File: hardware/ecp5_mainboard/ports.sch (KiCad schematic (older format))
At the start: 97 parts, among them J13 Micro_SD_Card, J3 HDMI_A, J4 USB_A, P4 JK0654219NL, U17 TPS2041B, U18 PCA9306, U19 TFP410, U20 TPS2041B, U21 KSZ9031RNXCA, U22 USB3300-EZK, Y2 25MHz, Y3 24MHz

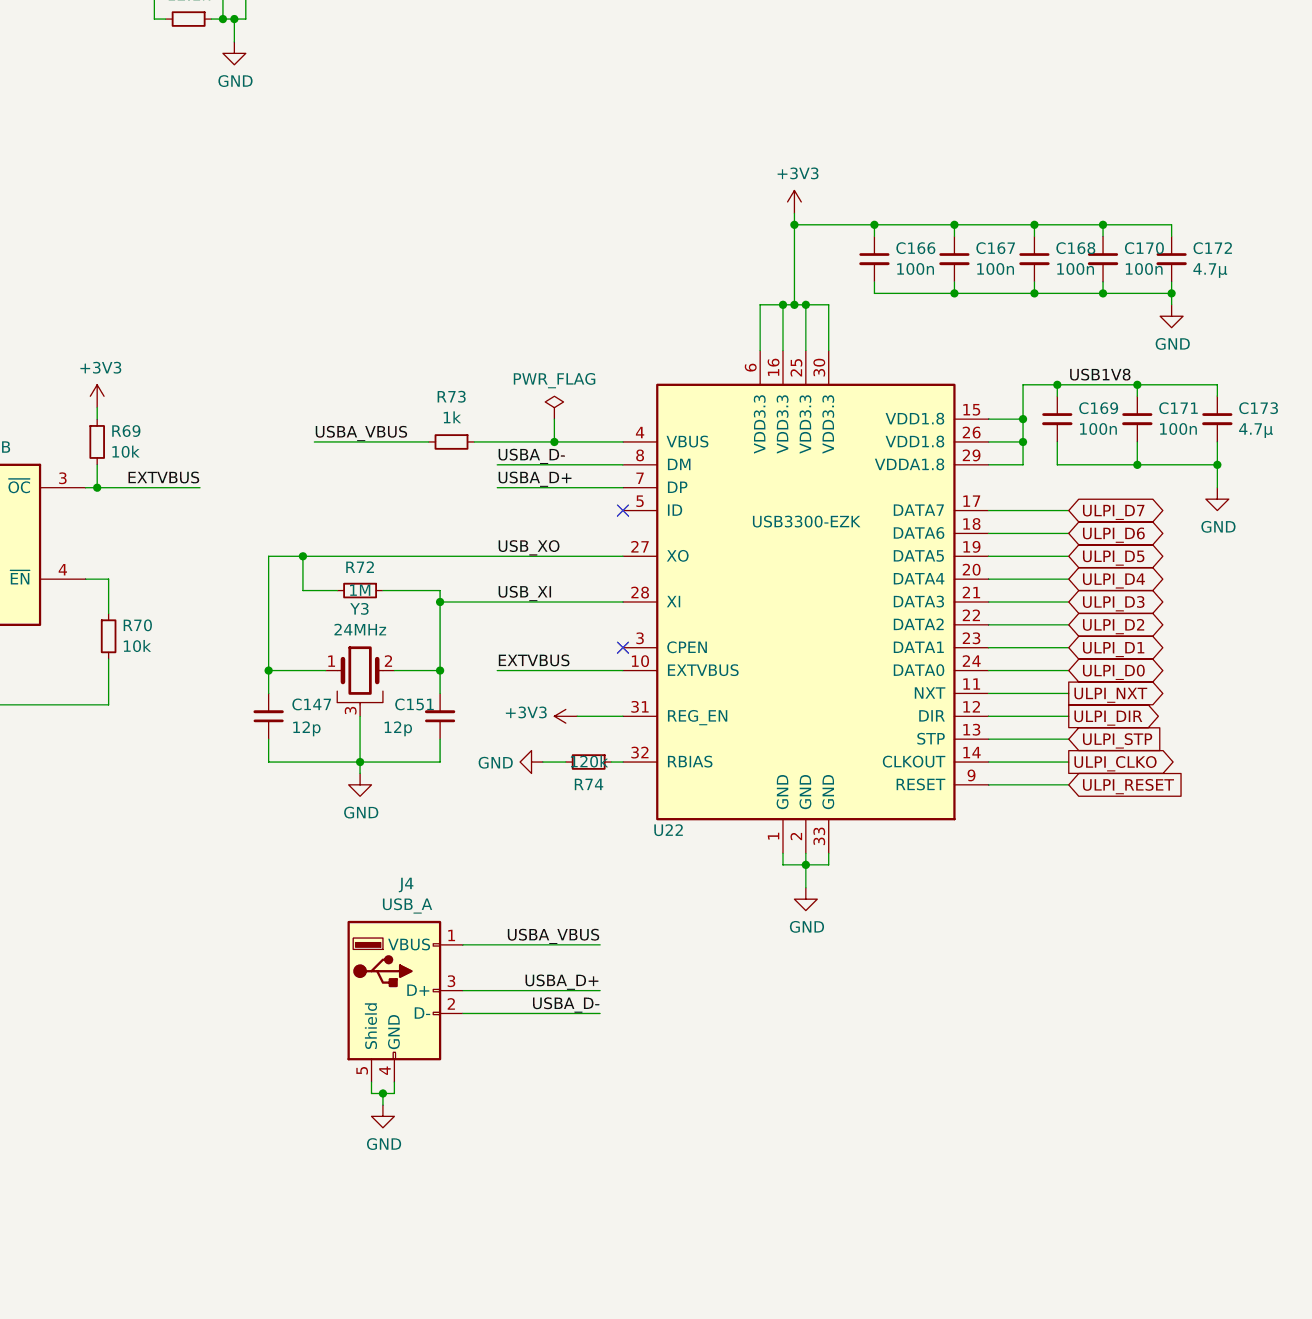
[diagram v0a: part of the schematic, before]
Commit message: hardware/mainboard: ERC fixes
Signed-off-by: David Shah <dave@ds0.me>
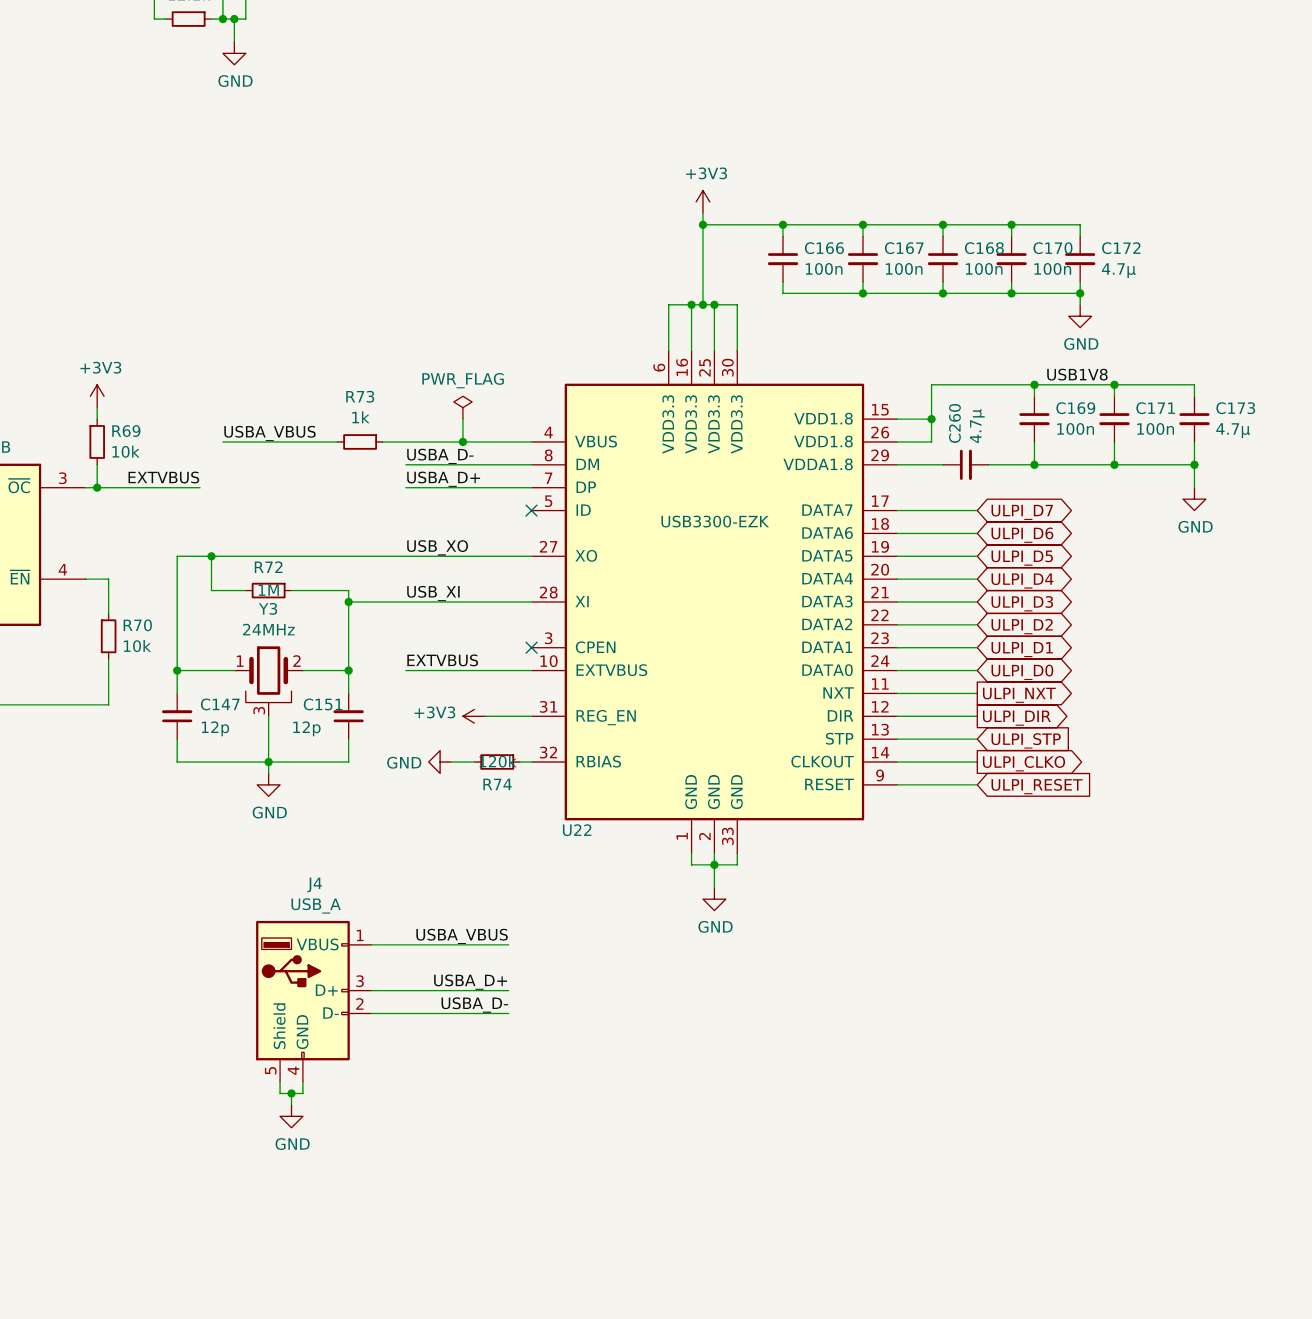
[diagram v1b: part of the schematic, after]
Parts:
- added C260: 4.7µ, Capacitor_SMD:C_0603_1608Metric, symbol Device:C_Small
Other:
- moved on the sheet: C147, C151, C166, C167, C168, C169, C170, C171, C172, C173, J4, R72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

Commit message: hardware/mainboard: BoM fixes, add USB power option
Signed-off-by: David Shah <dave@ds0.me>
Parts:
- J13: symbol Connector:Micro_SD_Card -> ecp5_mainboard-rescue:Micro_SD_Card-Connector
- U21: symbol Interface_Ethernet:KSZ9031RNXCA -> ecp5_mainboard-rescue:KSZ9031RNXCA-Interface_Ethernet
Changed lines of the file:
@@
 EESchema Schematic File Version 4
 LIBS:ecp5_mainboard-cache
-EELAYER 26 0
+EELAYER 29 0
 EELAYER END
 $Descr A3 16535 11693
@@
 $EndDescr
 $Comp
-L Interface_Ethernet:KSZ9031RNXCA U21
+L ecp5_mainboard-rescue:KSZ9031RNXCA-Interface_Ethernet U21
 U 1 1 5CA0A635
 P 11450 3250
@@
 	13650 750  14000 750
 $Comp
-L Connector:Micro_SD_Card J13
+L ecp5_mainboard-rescue:Micro_SD_Card-Connector J13
 U 1 1 632D42B7
 P 1550 1550
+AR Path="/632D42B7" Ref="J13"  Part="1"
+AR Path="/5CA09014/632D42B7" Ref="J13"  Part="1"
 F 0 "J13" H 1500 2267 50  0000 C CNN
 F 1 "Micro_SD_Card" H 1500 2176 50  0000 C CNN
